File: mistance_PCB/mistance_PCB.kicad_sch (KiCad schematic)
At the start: 22 parts, among them J1 USB_B_Micro, Q1 Q_PMOS_DSG, U1 ESP32-WROOM-32E, U2 TPS61200DRC, U3 MCP73831-2-OT, U4 AMS1117-3.3

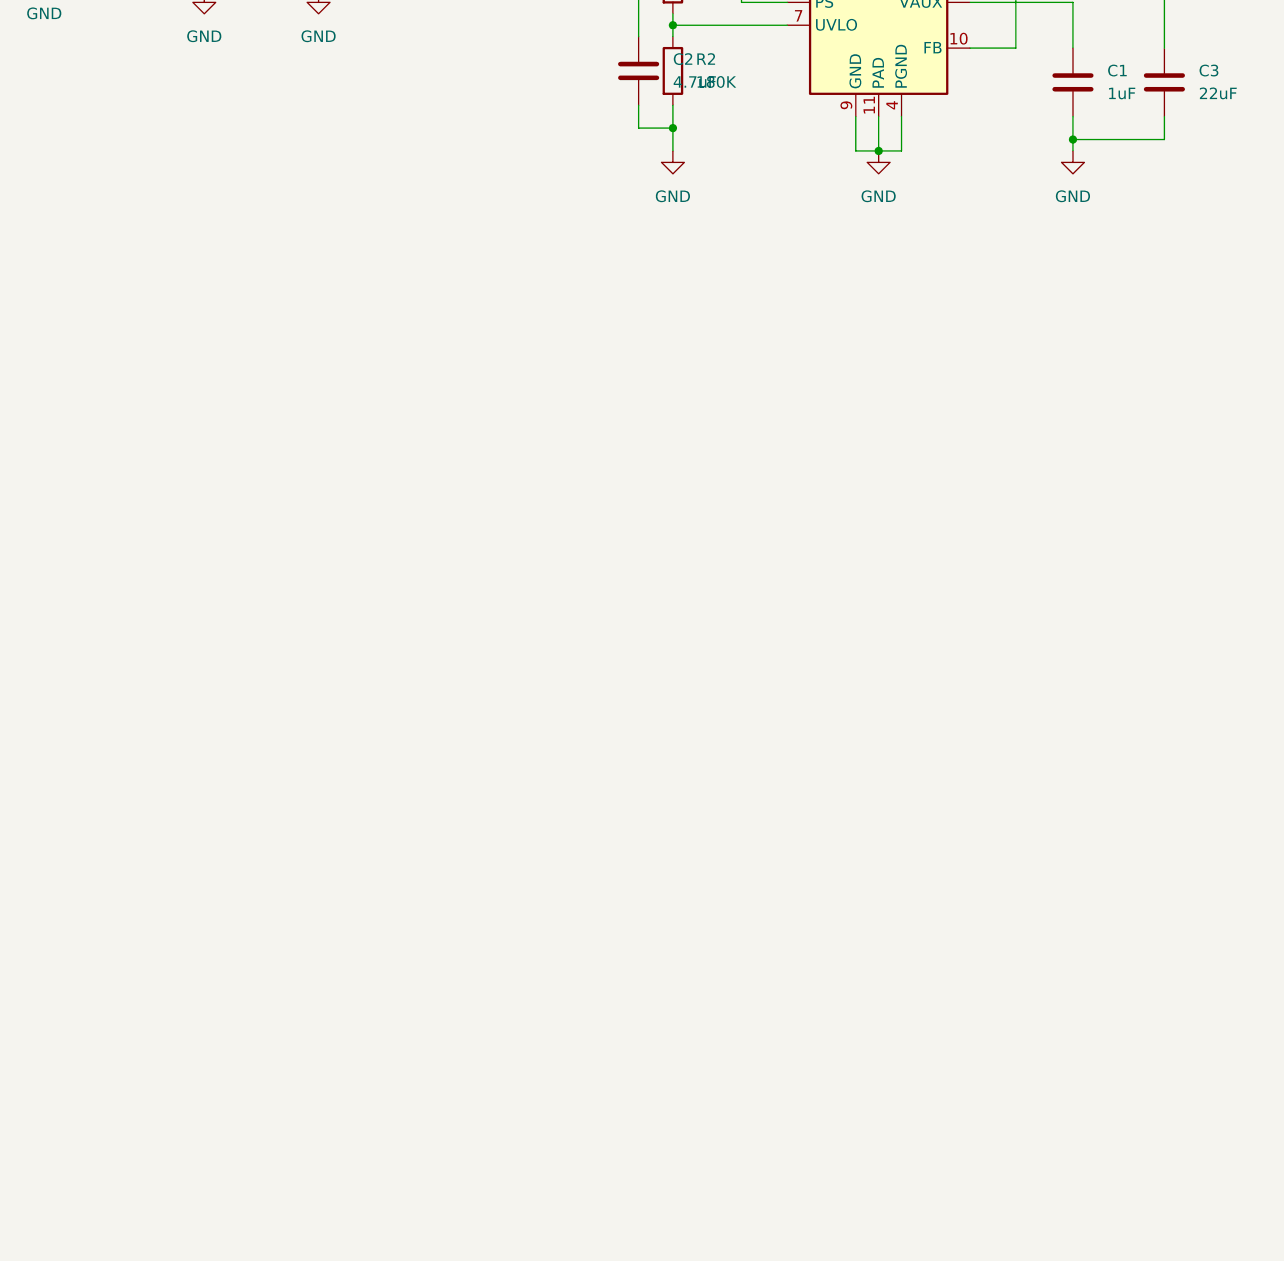
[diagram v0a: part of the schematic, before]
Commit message: PCB update
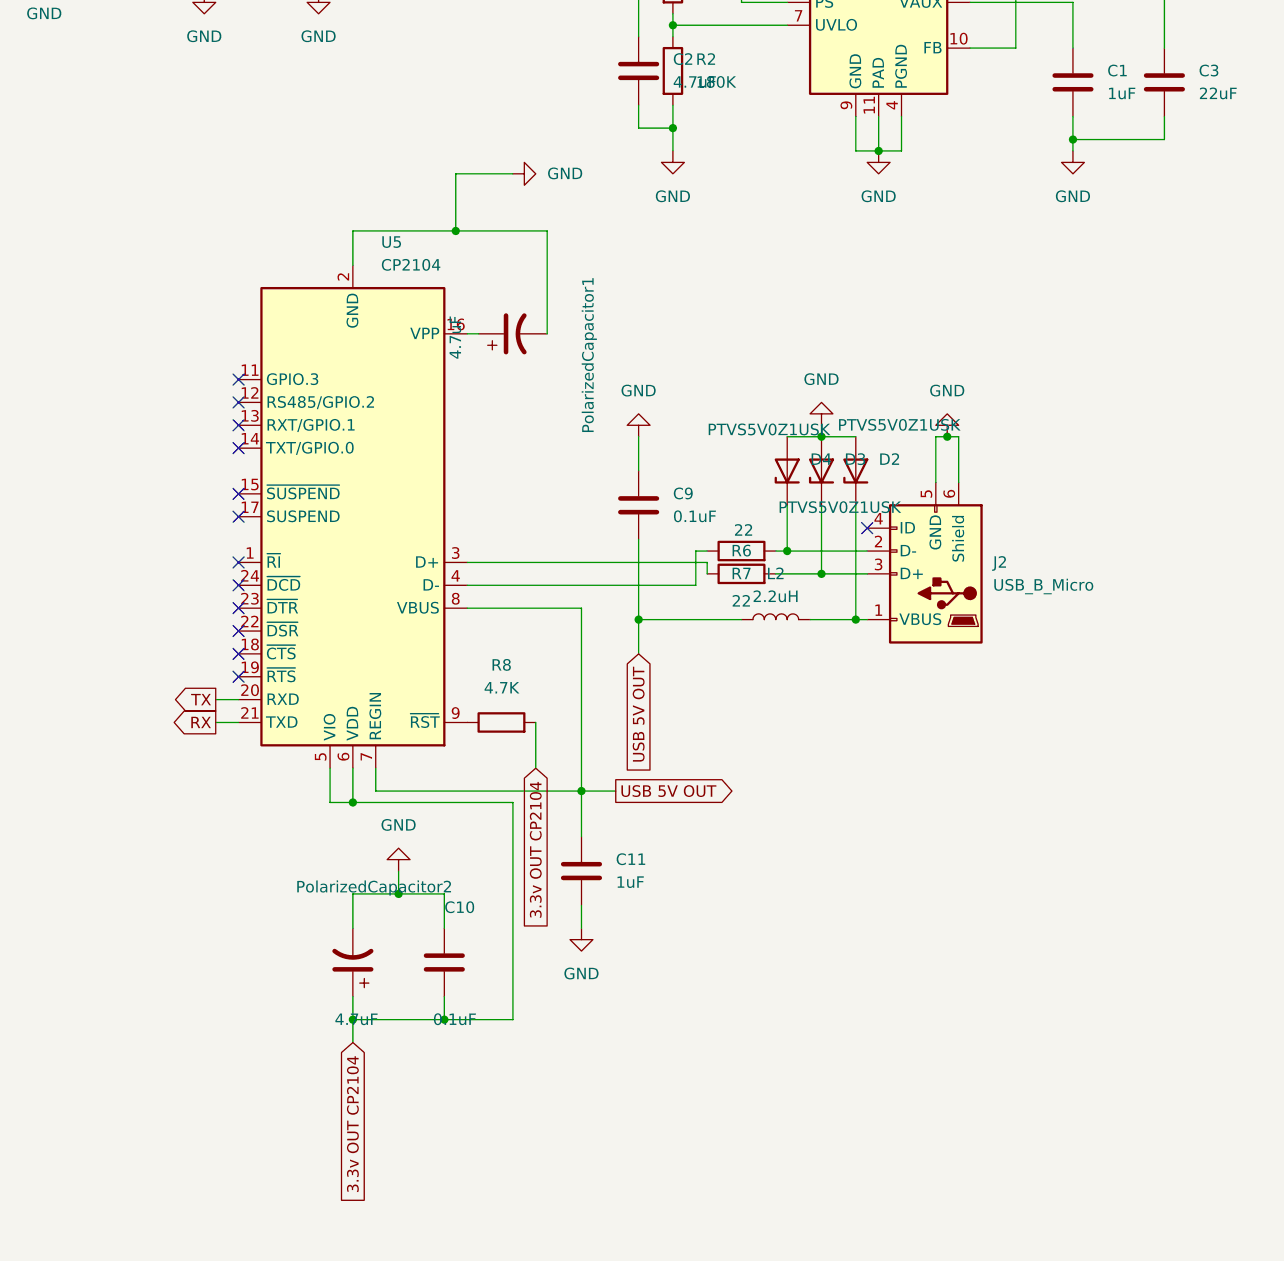
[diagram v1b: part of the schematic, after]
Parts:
- added C10, C9: 0.1uF, Capacitor_SMD:C_1210_3225Metric, symbol Device:C
- added C11: 1uF, Capacitor_SMD:C_1210_3225Metric, symbol Device:C
- added D2, D3, D4: PTVS5V0Z1USK, Diode_SMD:D_01005_0402Metric, symbol Diode:PTVS5V0Z1USK
- added J2: USB_B_Micro, Connector_USB:USB_Micro-B_Amphenol_10103594-0001LF_Horizontal, symbol Connector:USB_B_Micro
- added L2: 2.2uH, Inductor_SMD:L_1210_3225Metric, symbol Device:L
- added PolarizedCapacitor1, PolarizedCapacitor2: 4.7uF, Capacitor_SMD:C_1210_3225Metric, symbol Device:C_Polarized_US
- added R6, R7: 22, Resistor_SMD:R_0603_1608Metric, symbol Device:R
- added R8: 4.7K, Resistor_SMD:R_0603_1608Metric, symbol Device:R
- added U5: CP2104, Package_DFN_QFN:QFN-24-1EP_4x4mm_P0.5mm_EP2.6x2.6mm, symbol Interface_USB:CP2104
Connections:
- net GND: now also C10.1, C11.2, C9.1, D2.2 (A), D3.2 (A), D4.2 (A), J2.5 (GND), J2.6 (Shield), PolarizedCapacitor1.2, PolarizedCapacitor2.2, U5.2 (GND), U5.25 (GND)
- net RX: now also U5.21 (TXD)
- net TX: now also U5.20 (RXD)
- new net: PolarizedCapacitor1.1, U5.16 (VPP)
- new net: D2.1 (K), J2.1 (VBUS), L2.2
- new net: D3.1 (K), J2.3 (D+), R7.2
- new net: R7.1, U5.3 (D+)
- new net: D4.1 (K), J2.2 (D-), R6.2
- new net: R6.1, U5.4 (D-)
- new net: R8.1, U5.9 (~{RST})
- new net 3.3v OUT CP2104: C10.2, PolarizedCapacitor2.1, R8.2, U5.5 (VIO), U5.6 (VDD)
- new net USB 5V OUT: C11.1, C9.2, L2.1, U5.7 (REGIN), U5.8 (VBUS)
- no-connect marks 1 -> 14

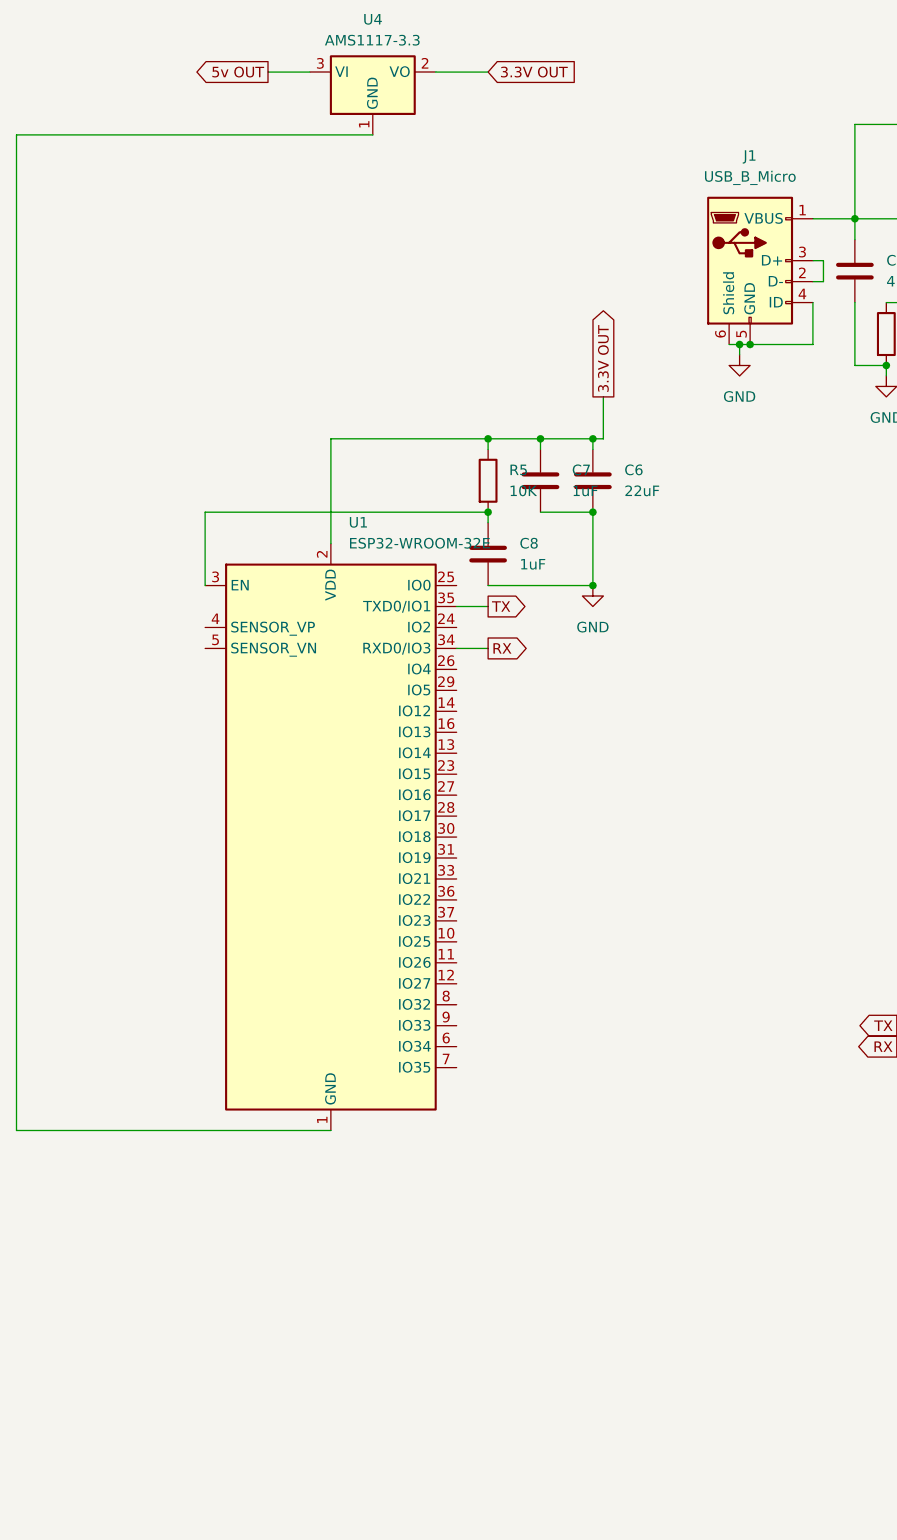
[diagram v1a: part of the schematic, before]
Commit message: PCB update
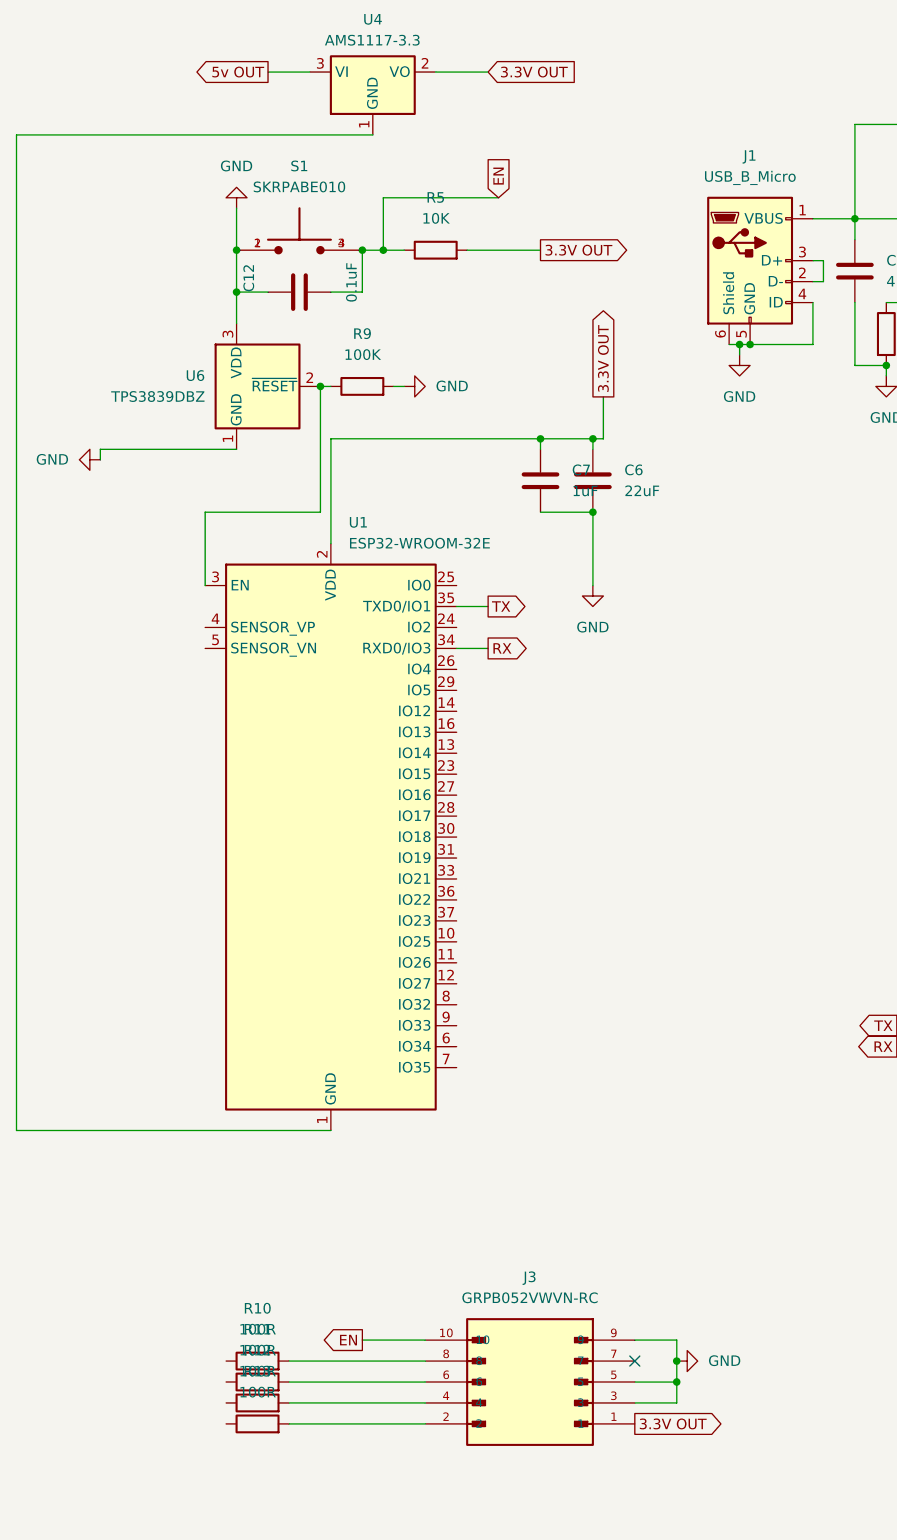
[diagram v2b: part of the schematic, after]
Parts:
- removed C8: 1uF, Capacitor_SMD:C_1210_3225Metric, symbol Device:C
- added C12: 0.1uF, Capacitor_SMD:C_1210_3225Metric, symbol Device:C
- added J3: GRPB052VWVN-RC, Varistor:SULLINS_GRPB052VWVN-RC, symbol GRPB052VWVN-RC:GRPB052VWVN-RC
- added R10, R11, R12, R13: 100R, Resistor_SMD:R_0603_1608Metric, symbol Device:R
- added R9: 100K, Resistor_SMD:R_0603_1608Metric, symbol Device:R
- added S1: SKRPABE010, SKRPABE010:SW_SKRPABE010, symbol SKRPABE010:SKRPABE010
- added U6: TPS3839DBZ, Package_TO_SOT_SMD:SOT-23, symbol Power_Supervisor:TPS3839DBZ
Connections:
- net 3.3V OUT: now also R5.2, J3.1; no longer R5.1
- net GND: now also C12.1, J3.3, J3.5, J3.9, R9.2, S1.1, S1.2, U6.1 (GND), U6.3 (VDD)
- net at U1.3 (EN): now also R9.1, U6.2 (~{RESET}); no longer R5.2
- new net: J3.8, R10.2
- new net: J3.6, R11.2
- new net: J3.2, R13.2
- new net: J3.4, R12.2
- new net EN: C12.2, J3.10, R5.1, S1.3, S1.4
- no-connect marks 14 -> 15
